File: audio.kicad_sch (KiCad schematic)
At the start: 57 parts, among them IC1 TAC5212IRGER, J13 Headphones 3.5mm, J18 Jack 6.35mm, J19 Jack 6.35mm, J20 Jack 6.35mm, J22 Jack 6.35mm, U14 OPA1656ID

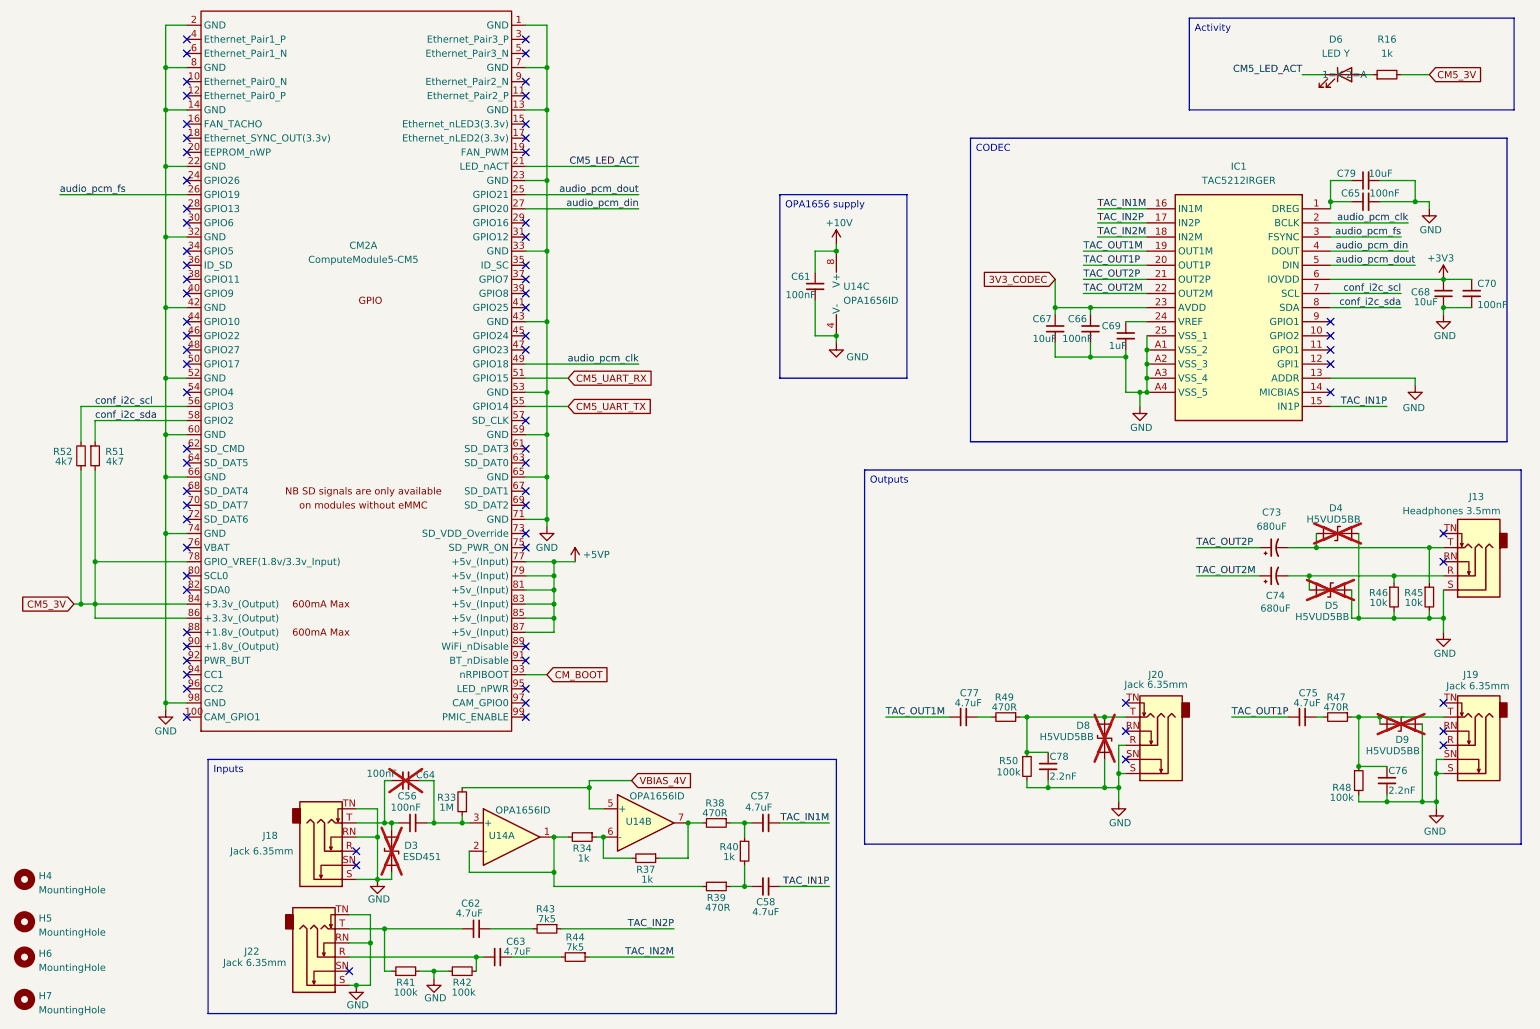
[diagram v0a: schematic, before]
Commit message: edited metadata
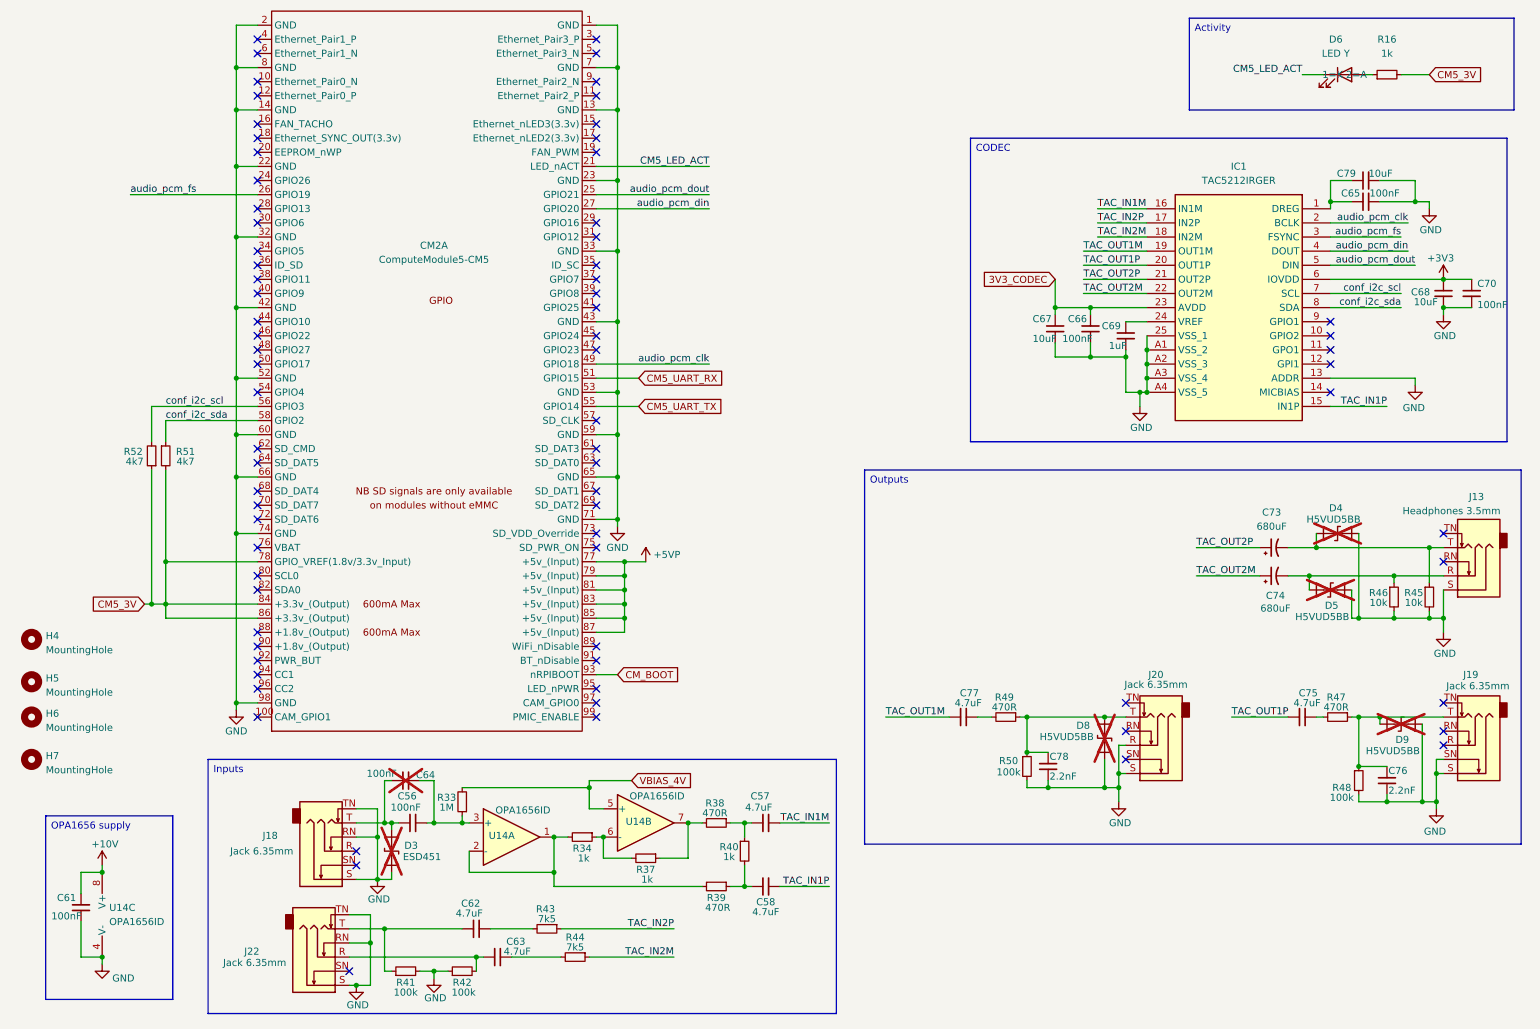
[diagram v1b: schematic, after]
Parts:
- IC1: Height 1 -> (none); JLCPCB part (none) -> C44853694; Manufacturer (none) -> Texas Instruments; Manufacturer part (none) -> TAC5212IRGER; Manufacturer_Name Texas Instruments -> (none); Manufacturer_Part_Number TAC5212IRGER -> (none); Notes (none) -> ADC1/2: differential AC-coupled, 5k/pin, 2Vrms differential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
- U14: JLCPCB part (none) -> C1346368; Manufacturer (none) -> Texas Instruments; Manufacturer part (none) -> OPA1656ID
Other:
- moved on the sheet: C61, CM2A, H4, H5, H6, H7, R51, R52, U14C
